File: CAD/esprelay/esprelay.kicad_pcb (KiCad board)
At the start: 2 copper layers, 65 x 20 mm, 42 parts, among them J1 Conn_01x06_Pin, J2 Conn_01x14_Pin, K1 G6K-2P-Y, K2 G6K-2P-Y, K3 G6K-2P-Y, Q1 Q_Photo_NPN, SW1 SW_SPST, U1 SPX3819M5-L-5-0, U2 SPX3819M5-L-3-3, U3 ESP-12F, U4 SHTC3, U5 ULN2003A

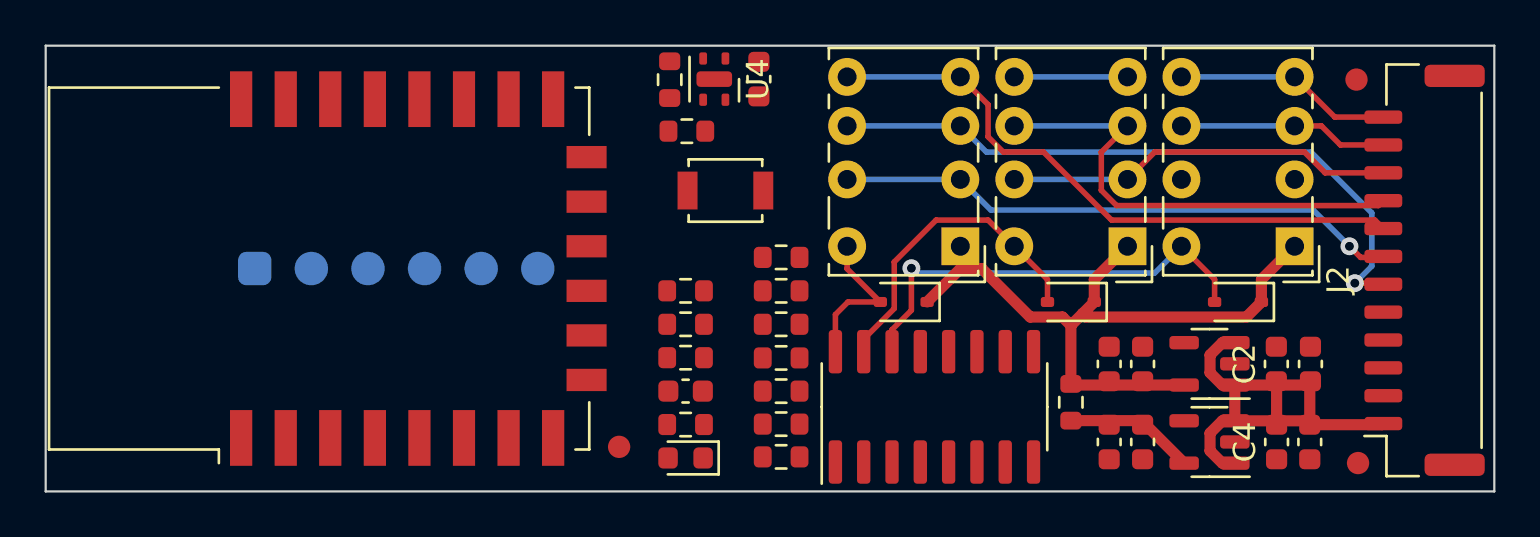
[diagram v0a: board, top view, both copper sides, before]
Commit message: Feat: Pretty much complete
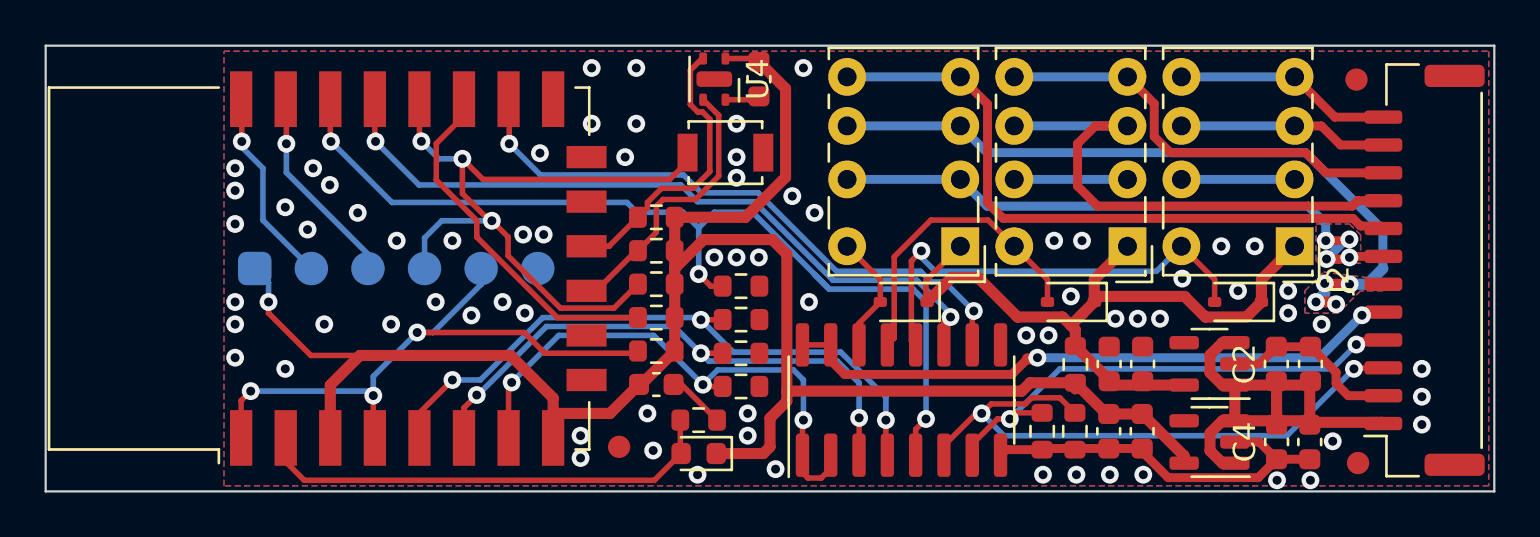
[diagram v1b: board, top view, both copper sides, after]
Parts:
- removed R11: 10K, Resistor_SMD:R_0603_1608Metric
- moved R13 13.2 mm to (146.2, 89.8), turned to -90 degrees
- moved R12 11.7 mm to (144.7, 89.8), turned to -90 degrees
- moved R5 6.20 mm to (127.4, 80.2), turned to 180 degrees
- moved R7 6.06 mm to (131.2, 87.8)
- moved R4 5.54 mm to (127.4, 81.7), turned to 180 degrees
- moved R10 3.69 mm to (131.2, 83.3)
- moved R8 3.33 mm to (131.2, 86.3)
- moved R2 2.23 mm to (127.4, 83.2), turned to 180 degrees
- moved R9 1.81 mm to (131.2, 84.8)
- moved R3 1.78 mm to (127.4, 84.7)
- moved JP1 1.71 mm to (146.2, 86.8)
- moved SW1 1.70 mm to (130.5, 77.3)
- moved U5 1.51 mm to (138.4, 88.4)
- moved C3 1.35 mm to (127.4, 87.7)
- moved R1 1.35 mm to (127.4, 86.2)
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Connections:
- D1 pad 2: HRO1 -> RO1
- D2 pad 2: HRO2 -> RO2
- D3 pad 2: HRO3 -> RO3
- J2 pad 10: R2NC -> R2NO
- J2 pad 3: HPO45 -> HI1
- J2 pad 4: HI06 -> HI2
- J2 pad 5: HI07 -> HO1
- K1 pad 8: HRO1 -> RO1
- K2 pad 8: HRO2 -> RO2
- K3 pad 8: HRO3 -> RO3
- R10 pad 1: LPO4 -> GPIO5
- R12 pad 1: HI07 -> HI2
- R13 pad 1: HI06 -> HI1
- R7 pad 1: LRO1 -> GPIO13
- R8 pad 1: LRO2 -> GPIO12
- R9 pad 1: LR03 -> GPIO14
- U3 pad 16: LRO1 -> GPIO15
- U3 pad 19: LP45 -> GPIO4
- U3 pad 20: LI07 -> GPIO5
- U3 pad 5: LRO2 -> GPIO14
- U3 pad 6: LI06 -> GPIO12
- U3 pad 7: LR03 -> GPIO13
- U5 pad 1: LRO1 -> GPIO13
- U5 pad 10: LI07 -> GPIO15
- U5 pad 11: LI06 -> GPIO4
- U5 pad 12: HP45 -> RO3
- U5 pad 13: HP45 -> RO2
- U5 pad 14: HRO3 -> RO1
- U5 pad 15: HRO2 -> HO1
- U5 pad 16: HRO1 -> HO1
- U5 pad 2: LRO2 -> GPIO13
- U5 pad 3: LR03 -> GPIO12
- U5 pad 4: LP45 -> GPIO14
- U5 pad 5: LP45 -> GPIO5
- U5 pad 6: HI06 -> HI1
- U5 pad 7: HI07 -> HI2
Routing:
- net +3.3V: track 5.87 -> 86.6 mm, vias 0 -> 1
- net GPIO5: track 0.00 -> 43.6 mm, vias 0 -> 3
- net GPIO4: track 0.00 -> 32.7 mm, vias 0 -> 2
- net BOOT: track 0.00 -> 32.5 mm, vias 0 -> 3
- net GND: track 0.00 -> 29.5 mm, vias 0 -> 70
- net GPIO14: track 0.00 -> 28.9 mm, vias 0 -> 3
- net RST: track 0.00 -> 28.2 mm, vias 0 -> 3
- net HO1: track 0.00 -> 28.2 mm, vias 0 -> 2
- net GPIO15: track 0.00 -> 27.5 mm, vias 0 -> 2
- net HI1: track 0.00 -> 27.2 mm, vias 0 -> 2
- net GPIO12: track 0.00 -> 25.9 mm, vias 0 -> 3
- net GPIO13: track 0.00 -> 25.1 mm, vias 0 -> 3
- net HI2: track 0.00 -> 22.4 mm, vias 0 -> 2
- net PHOTO_OUT: track 0.00 -> 21.2 mm
- net RO3: track 0.00 -> 20.3 mm, vias 0 -> 1
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- added copper zone on B.Cu, net GND
- added copper zone on F.Cu, net GND
- added copper zone on B.Cu, net R1A
- added copper zone on F.Cu, net R1A
- added copper zone on B.Cu, net R1NC
- added copper zone on F.Cu, net R1NC
